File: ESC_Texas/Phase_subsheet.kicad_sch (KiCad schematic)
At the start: 12 parts, among them IC8 AD8411AWBRZ, J10 Conn_01x03_Pin, J9 Conn_01x03_Pin

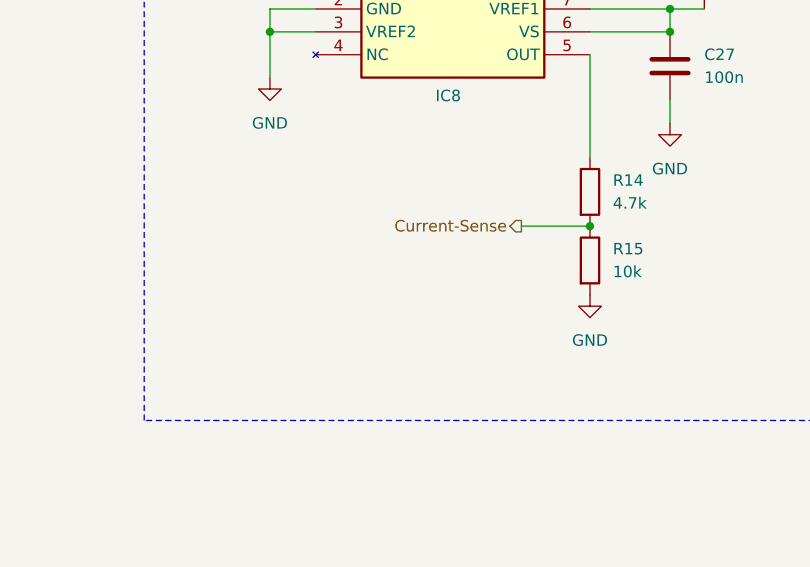
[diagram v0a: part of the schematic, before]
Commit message: filters
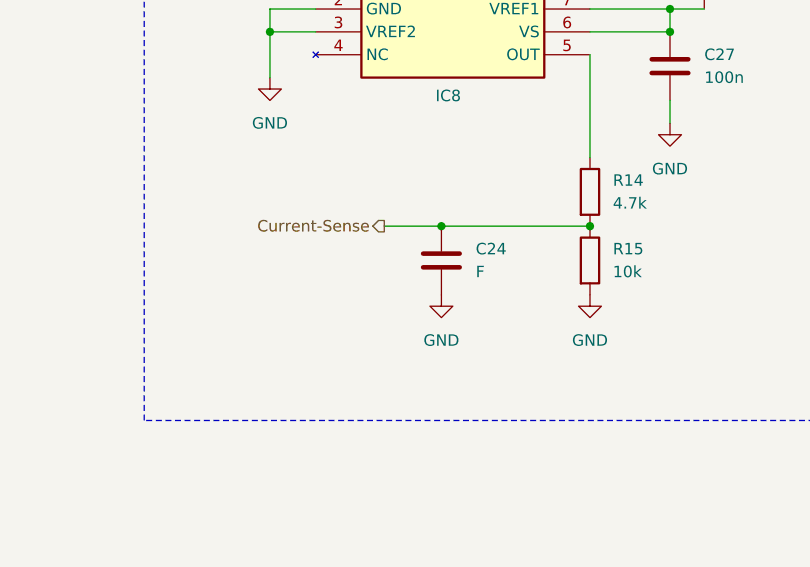
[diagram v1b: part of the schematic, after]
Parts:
- added C24: F, Capacitor_SMD:C_0805_2012Metric, symbol Device:C
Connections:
- net Current-Sense: now also C24.1
- net GND: now also C24.2
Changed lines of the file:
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@@
+	)
+	(junction
+		(at 166.37 134.62)
+		(diameter 0)
+		(color 0 0 0 0)
 	)
 	(junction
@@
 	(wire
 		(pts
-			(xy 175.26 134.62) (xy 182.88 134.62)
+			(xy 160.02 134.62) (xy 166.37 134.62)
 		)
 		(stroke
@@
 		(pts
 			(xy 182.88 115.57) (xy 182.88 127)
+		)
+		(stroke
+			(width 0)
+			(type default)
+		)
+	)
+	(wire
+		(pts
+			(xy 166.37 134.62) (xy 182.88 134.62)
 		)
 		(stroke
@@
 	(hierarchical_label "Current-Sense"
 		(shape output)
-		(at 175.26 134.62 180)
+		(at 160.02 134.62 180)
 		(fields_autoplaced yes)
 		(effects
@@
 	)
 	(symbol
+		(lib_id "Device:C")
+		(at 166.37 138.43 0)
+		(unit 1)
+		(exclude_from_sim no)
+		(in_bom yes)
+		(on_board yes)
+		(dnp no)
+		(fields_autoplaced yes)
+		(property "Reference" "C24"
+			(at 170.18 137.1599 0)
+			(effects
+				(font
+					(size 1.27 1.27)
+				)
+				(justify left)
+			)
+		)
+		(property "Value" "F"
+			(at 170.18 139.6999 0)
+			(effects
+				(font
+					(size 1.27 1.27)
+				)
+				(justify left)
+			)
+		)
+		(property "Footprint" "Capacitor_SMD:C_0805_2012Metric"
+			(at 167.3352 142.24 0)
+			(effects
+				(font
+					(size 1.27 1.27)
+				)
+				(hide yes)
+			)
+		)
+		(property "Datasheet" "~"
+			(at 166.37 138.43 0)
+			(effects
+				(font
+					(size 1.27 1.27)
+				)
+				(hide yes)
+			)
+		)
+		(property "Description" "Unpolarized capacitor"
+			(at 166.37 138.43 0)
+			(effects
+				(font
+					(size 1.27 1.27)
+				)
+				(hide yes)
+			)
+		)
+		(pin "2"
+		)
+		(pin "1"
+		)
+		(instances
+			(project "ESC_Texas"
+				(path "/0e3a5351-d2cd-4ecc-a1be-cca9c5f62ea0/553690e4-0a20-4b8e-821c-55ba3788d3c5"
+					(reference "C50")
+					(unit 1)
+				)
+				(path "/0e3a5351-d2cd-4ecc-a1be-cca9c5f62ea0/63c8dce8-451d-41ee-b438-d688cf3e64bd"
+					(reference "C29")
+					(unit 1)
+				)
+				(path "/0e3a5351-d2cd-4ecc-a1be-cca9c5f62ea0/b8e552f6-93a8-4098-a907-a65be165d984"
+					(reference "C24")
+					(unit 1)
+				)
+			)
+		)
+	)
+	(symbol
 		(lib_id "Device:R_US")
 		(at 152.4 92.71 0)
@@
 					(unit 1)
 				)
+			)
+		)
+	)
+	(symbol
+		(lib_id "power:GND")
+		(at 166.37 142.24 0)
+		(unit 1)
+		(exclude_from_sim no)
+		(in_bom yes)
+		(on_board yes)
+		(dnp no)
+		(fields_autoplaced yes)
+		(property "Reference" "#PWR045"
+			(at 166.37 148.59 0)
+			(effects
+				(font
+					(size 1.27 1.27)
+				)
+				(hide yes)
+			)
+		)
+		(property "Value" "GND"
+			(at 166.37 147.32 0)
+			(effects
+				(font
+					(size 1.27 1.27)
+				)
+			)
+		)
+		(property "Footprint" ""
+			(at 166.37 142.24 0)
+			(effects
+				(font
+					(size 1.27 1.27)
+				)
+				(hide yes)
+			)
+		)
+		(property "Datasheet" ""
+			(at 166.37 142.24 0)
+			(effects
+				(font
+					(size 1.27 1.27)
+				)
+				(hide yes)
+			)
+		)
+		(property "Description" "Power symbol creates a global label with name \"GND\" , ground"
+			(at 166.37 142.24 0)
+			(effects
+				(font
+					(size 1.27 1.27)
+				)
+				(hide yes)
+			)
+		)
+		(pin "1"
+		)
+		(instances
+			(project "ESC_Texas"
+				(path "/0e3a5351-d2cd-4ecc-a1be-cca9c5f62ea0/553690e4-0a20-4b8e-821c-55ba3788d3c5"
+					(reference "#PWR047")
+					(unit 1)
+				)
+				(path "/0e3a5351-d2cd-4ecc-a1be-cca9c5f62ea0/63c8dce8-451d-41ee-b438-d688cf3e64bd"
+					(reference "#PWR046")
+					(unit 1)
+				)
+				(path "/0e3a5351-d2cd-4ecc-a1be-cca9c5f62ea0/b8e552f6-93a8-4098-a907-a65be165d984"
+					(reference "#PWR045")
+					(unit 1)
+				)
